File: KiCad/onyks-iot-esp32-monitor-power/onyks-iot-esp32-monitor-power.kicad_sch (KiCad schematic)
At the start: 19 parts, among them J1 Uart_con, J2 Jtag_con, SW1 reset, U1 ESP32-WROOM-32D, U2 ADS1115IDGS, U3 ACS712xLCTR-30A

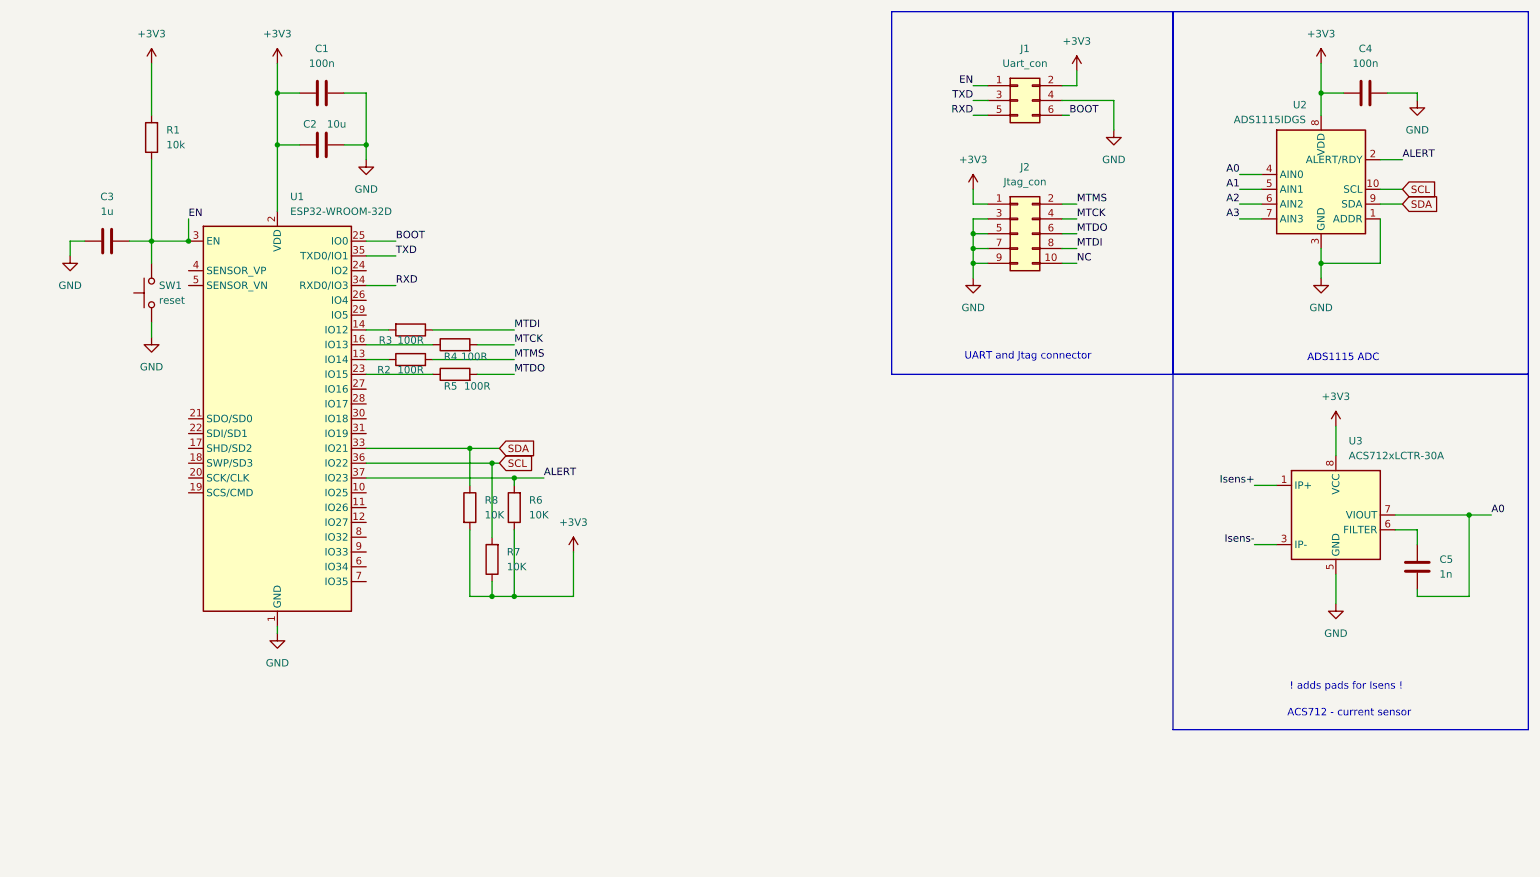
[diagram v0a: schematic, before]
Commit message: edit schemat
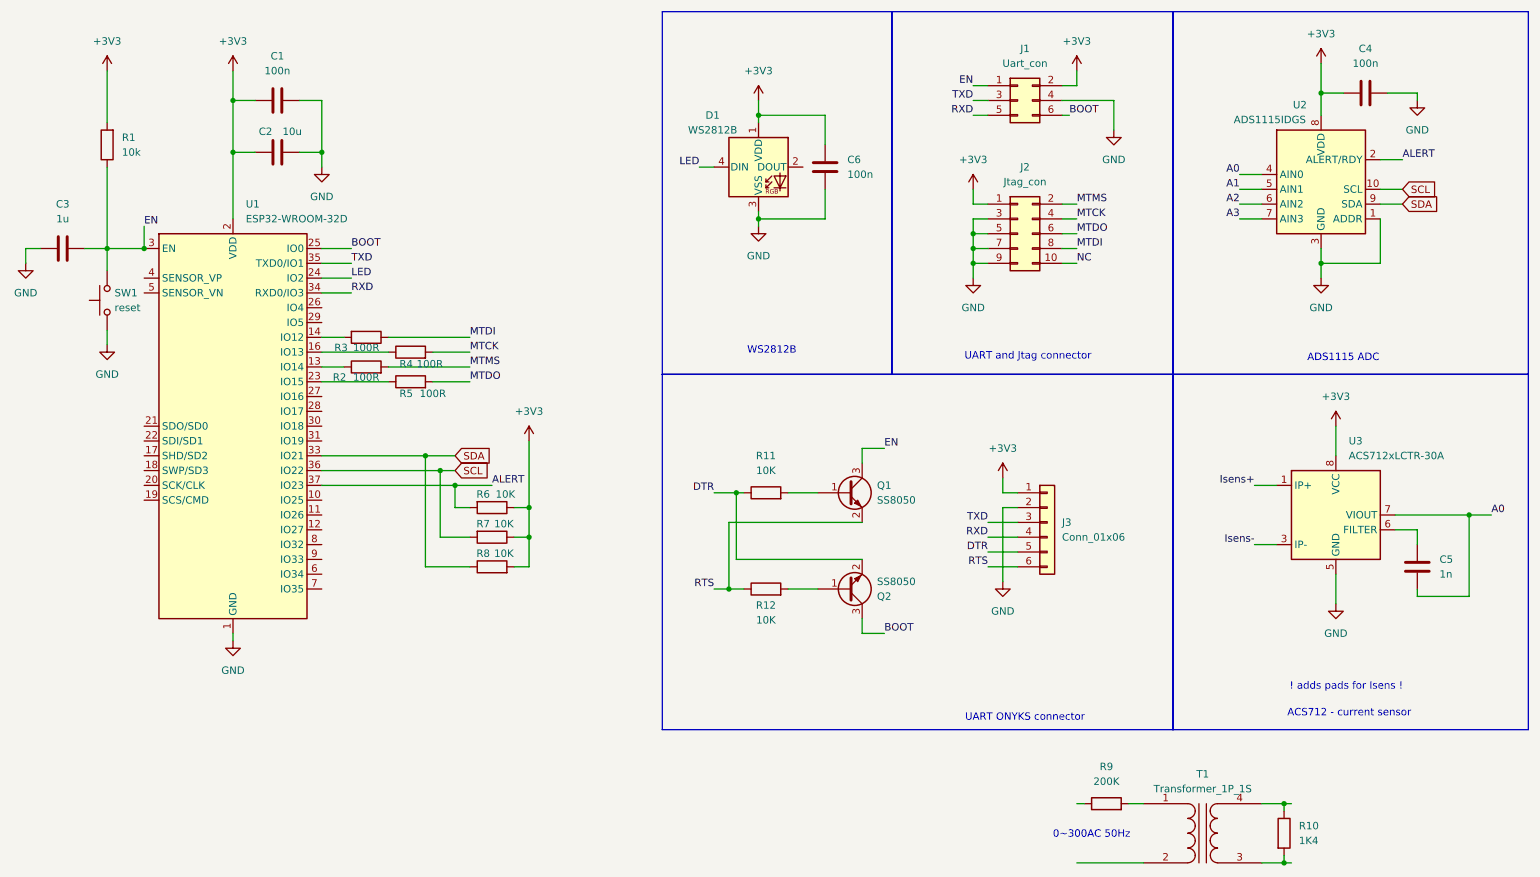
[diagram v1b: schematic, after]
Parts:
- added C6: 100n, symbol Device:C
- added D1: WS2812B, LED_SMD:LED_WS2812B_PLCC4_5.0x5.0mm_P3.2mm, symbol LED:WS2812B
- added J3: Conn_01x06, Connector_PinHeader_2.54mm:PinHeader_1x06_P2.54mm_Vertical, symbol Connector_Generic:Conn_01x06
- added Q1: SS8050, Package_TO_SOT_SMD:SOT-23-3, symbol Transistor_BJT:SS8050
- added Q2: SS8050, Package_TO_SOT_SMD:SOT-23, symbol Transistor_BJT:SS8050
- added R10: 1K4, symbol Device:R
- added R11, R12: 10K, symbol Device:R
- added R9: 200K, symbol Device:R
- added T1: Transformer_1P_1S, symbol Device:Transformer_1P_1S
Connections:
- net +3V3: now also C6.1, D1.1 (VDD), J3.1 (Pin_1)
- net BOOT: now also Q2.3 (C)
- net EN: now also Q1.3 (C)
- net GND: now also C6.2, D1.3 (VSS), J3.2 (Pin_2)
- net RXD: now also J3.4 (Pin_4)
- net TXD: now also J3.3 (Pin_3)
- net LED: now reaches U1.24 (IO2)
- net LED: now also D1.4 (DIN)
- new net: R10.1, T1.4 (SB)
- new net: R10.2, T1.3 (SA)
- new net: Q1.1 (B), R11.2
- new net: R9.2, T1.1 (AA)
- new net: Q2.1 (B), R12.2
- new net DTR: J3.5 (Pin_5), Q2.2 (E), R11.1
- new net RTS: J3.6 (Pin_6), Q1.2 (E), R12.1
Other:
- note added: "0~300AC 50Hz"
- note added: "UART ONYKS connector"
- note added: "WS2812B"
- moved on the sheet: C1, C2, C3, R1, R2, R3, R4, R5, R6, R7, R8, SW1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
